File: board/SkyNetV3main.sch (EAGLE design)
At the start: 67 parts, among them IC1 HC_05, IC2 RF4463PRO, IC3 LPC1768, IC4 BCX17, IC5 TPS63001, IC6 MCP73871-2CCI/ML, Q1 32.768KHz, Q2 12MHz, Q3 IRLM6402, Q4 BSS138, X1 BAT

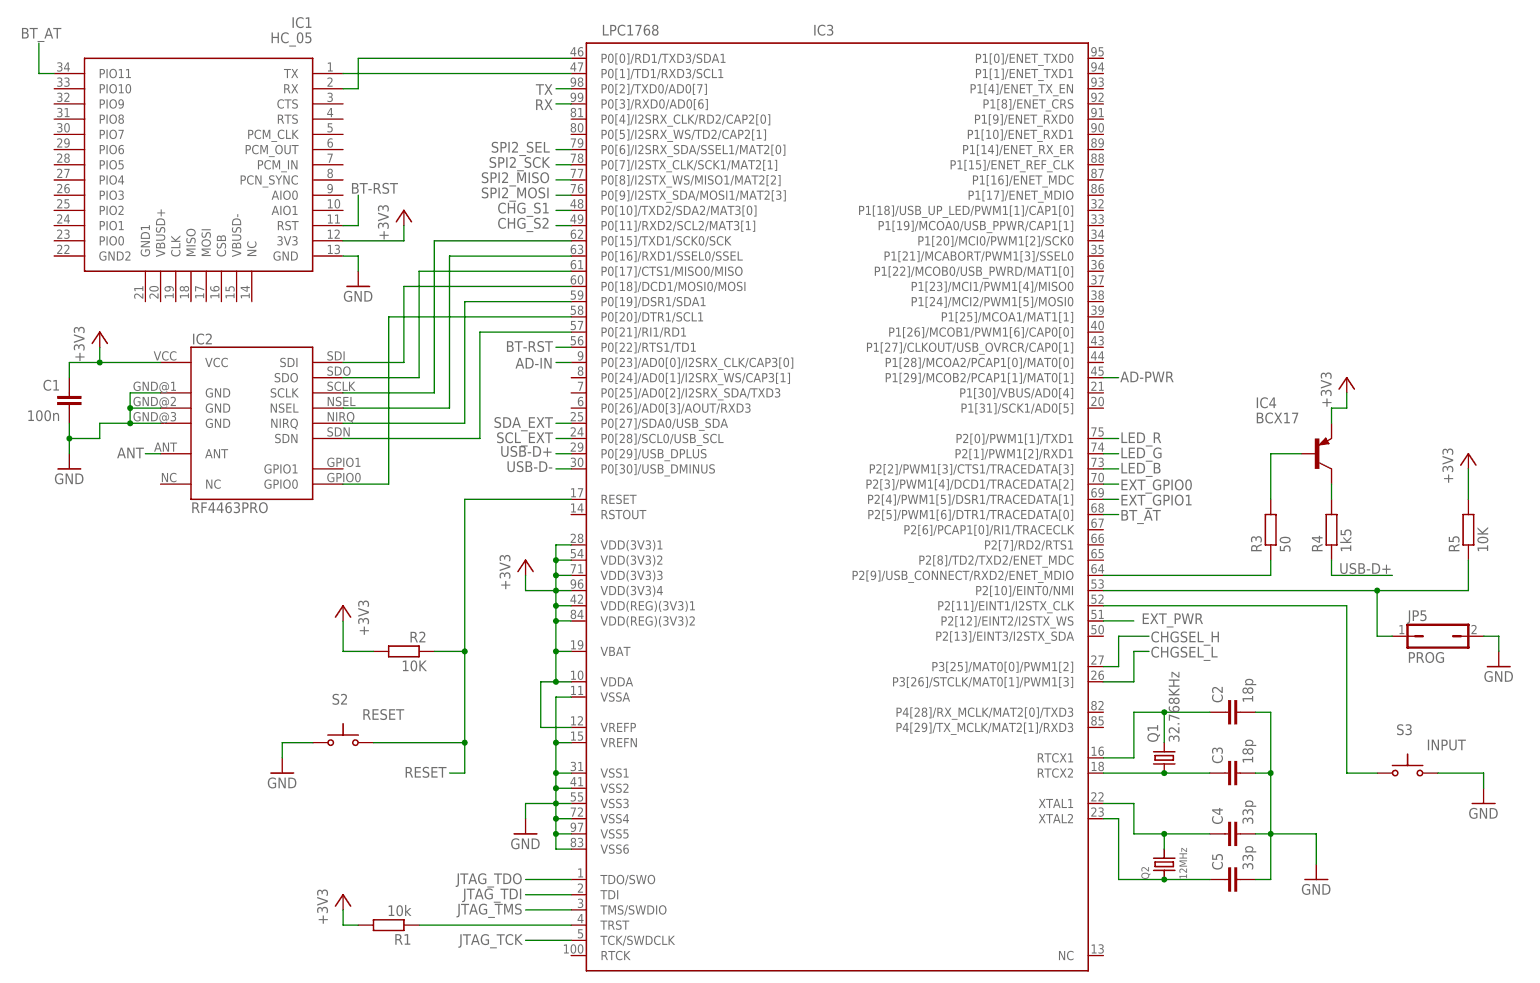
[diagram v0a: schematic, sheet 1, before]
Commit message: new layout
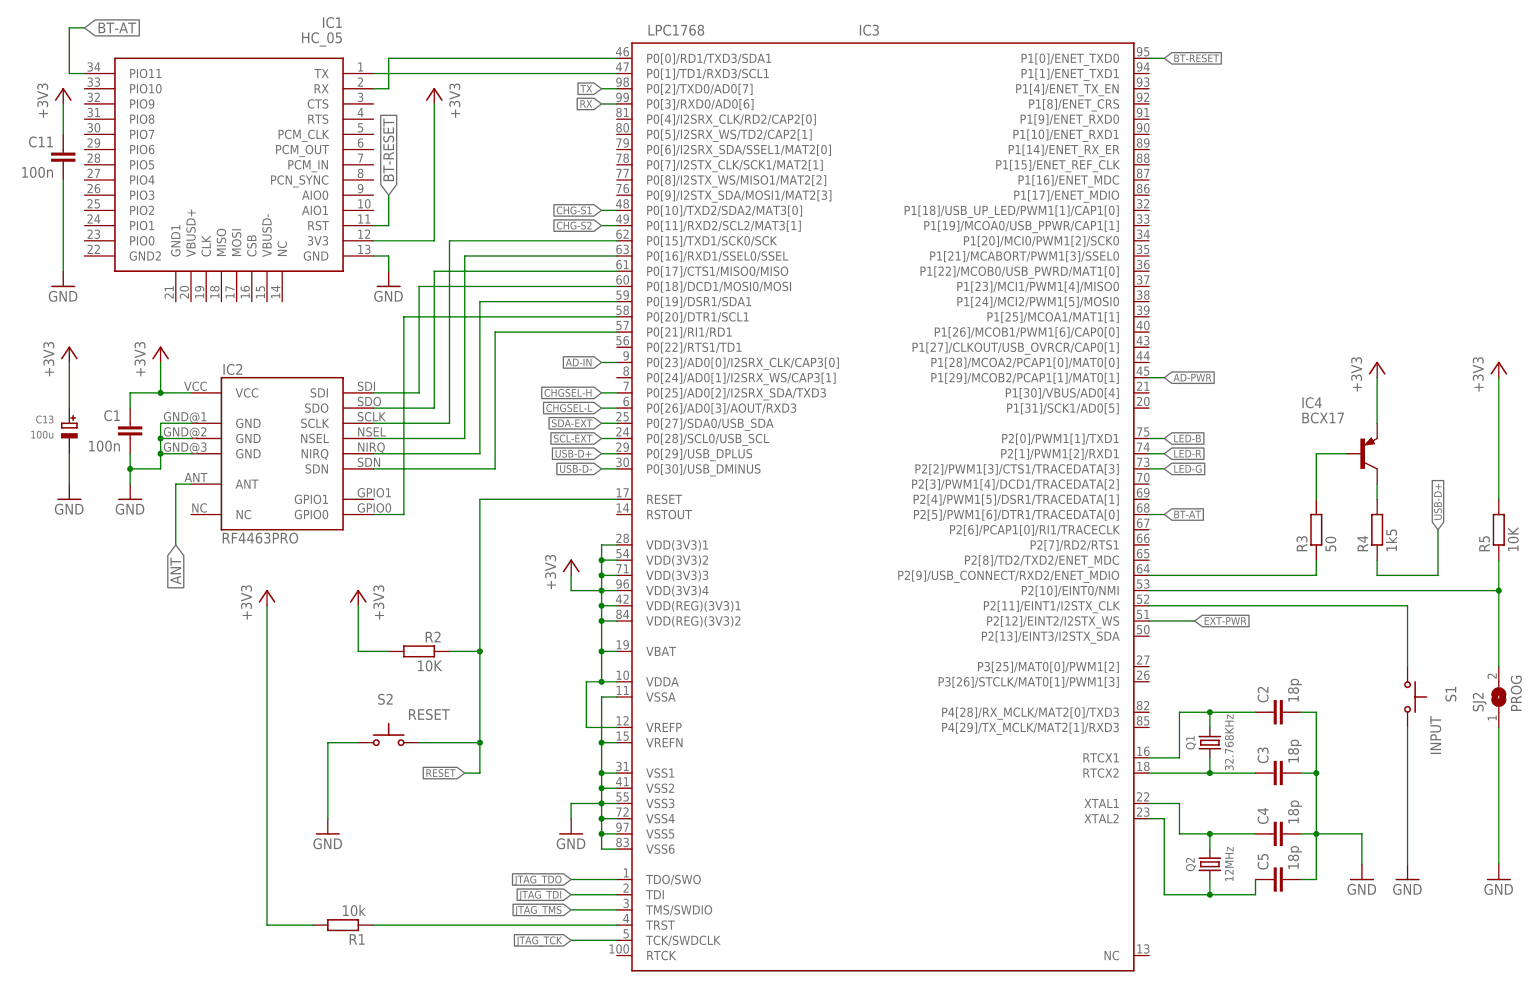
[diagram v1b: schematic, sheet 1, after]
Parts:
- removed C14: 100n, rcl:C-EUC0603
- removed JP1: MEASURE, jumper:JP1Q
- removed JP2: DEBUG, pinhead:PINHD-1X5
- removed JP4: PERIPH, microbuilder:HEADER-2X51.27MM
- removed JP5: PROG, jumper:JP1Q
- removed LED1: STATUS, skynet_other:RGB-LED
- removed OK1, OK2, OK3: PC3H7, skynet_other:PC3H7
- removed R7, R8: 91, rcl:R-EU_R0603
- removed S3: INPUT, skynet_other:PT645VERT
- added D1: 3v3, diode:ZENER-DIODESOT23
- added LED2: RGBLED5050, adafruit:RGBLED5050
- added S1: INPUT, switch-ck:PTS645SSMTR
- added SJ1: (no value), jumper:SJ
- added SJ2: PROG, jumper:SJ
- added U$2: (no value), skynet_other:PIN-HEAD-1X3
- C12, C13: value 100n -> 100u; device rcl:C-EUC0603 -> microbuilder:CAP_TANTALUMC/6032_WAVE
- C4, C5: value 33p -> 18p
- Q1: device crystal-2:CRYSTALMM20SS -> skynet_other:XTAL2-PAD
- Q2: device microbuilder:CRYSTALSMD -> skynet_other:XTAL4-PAD
- R6: value 91 -> 10k
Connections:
- net BT_AT renamed BT-AT
- net BT_RX renamed BT-RX
- net BT_TX renamed BT-TX
- net RTCX2 renamed N$2
- net SDI renamed RF-SDI
- net SPI0-NIRQ renamed RF-NIRQ
- net SPI0-NSEL renamed RF-NSEL
- net SPI0-SCLK renamed RF-SCLK
- net SPI0-SDN renamed RF-SDN
- net SPI0-SDO renamed RF-SDO
- removed net BT-RST: IC1.RST, IC3.P0[22]/RTS1/TD1
- removed net CHGSEL_H: IC3.P3[25]/MAT0[0]/PWM1[2], IC6.SEL
- removed net CHGSEL_L: IC3.P3[26]/STCLK/MAT0[1]/PWM1[3], IC6.PROG2
- removed net CHG_S1: IC3.P0[10]/TXD2/SDA2/MAT3[0], OK3.COL
- removed net CHG_S2: IC3.P0[11]/RXD2/SCL2/MAT3[1], OK2.COL
- removed net EXT_GPIO0: IC3.P2[3]/PWM1[4]/DCD1/TRACEDATA[2], JP4.6
- removed net EXT_GPIO1: IC3.P2[4]/PWM1[5]/DSR1/TRACEDATA[1], JP4.8
- removed net EXT_PWR: IC3.P2[12]/EINT2/I2STX_WS, OK1.COL
- removed net LED_B: IC3.P2[2]/PWM1[3]/CTS1/TRACEDATA[3], LED1-B.C
- removed net LED_G: IC3.P2[1]/PWM1[2]/RXD1, LED1-G.C
- removed net LED_R: IC3.P2[0]/PWM1[1]/TXD1, LED1-R.C
- removed net PG: IC6./PG, R6.1
- removed net PG-OK: OK1.C, R6.2
- removed net SCL_EXT: IC3.P0[28]/SCL0/USB_SCL, JP4.4
- removed net SDA_EXT: IC3.P0[27]/SDA0/USB_SDA, JP4.2
- removed net SPI2_MISO: IC3.P0[8]/I2STX_WS/MISO1/MAT2[2], JP4.5
- removed net SPI2_MOSI: IC3.P0[9]/I2STX_SDA/MOSI1/MAT2[3], JP4.7
- removed net SPI2_SCK: IC3.P0[7]/I2STX_CLK/SCK1/MAT2[1], JP4.3
- removed net SPI2_SEL: IC3.P0[6]/I2SRX_SDA/SSEL1/MAT2[0], JP4.1
- removed net STAT1: IC6.STAT1/LBO, R8.1
- removed net STAT1-OK: OK3.C, R8.2
- removed net STAT2: IC6.STAT2, R7.1
- removed net STAT2-OK: OK2.C, R7.2
- new net BT-RESET: IC1.RST, IC3.P1[0]/ENET_TXD0
- new net CHG-S1: IC3.P0[10]/TXD2/SDA2/MAT3[0], IC6.STAT1/LBO
- new net CHG-S2: IC3.P0[11]/RXD2/SCL2/MAT3[1], IC6.STAT2
- new net CHGSEL-H: IC3.P0[25]/AD0[2]/I2SRX_SDA/TXD3, IC6.SEL
- new net CHGSEL-L: IC3.P0[26]/AD0[3]/AOUT/RXD3, IC6.PROG2
- new net EXT-PWR: D1.C, IC3.P2[12]/EINT2/I2STX_WS, R6.2
- new net LED-B: IC3.P2[0]/PWM1[1]/TXD1, LED2.BLUE_C
- new net LED-G: IC3.P2[2]/PWM1[3]/CTS1/TRACEDATA[3], LED2.GREEN_C
- new net LED-R: IC3.P2[1]/PWM1[2]/RXD1, LED2.RED_C
- new net SCL-EXT: IC3.P0[28]/SCL0/USB_SCL, U$2.4
- new net SDA-EXT: IC3.P0[27]/SDA0/USB_SDA, U$2.3
- net +3V3: now also C12.+, C13.+, U$2.5; no longer C12.1, C13.1, C14.1, JP2.4, JP4.10
- net +5V: now also R6.1; no longer OK1.A, OK2.A, OK3.A
- net GND: now also C12.-, C13.-, D1.A, S1.S, SJ2.1, U$2.6; no longer C12.2, C13.2, C14.2, JP2.5, JP4.9, JP5.2, OK1.EMI, OK2.EMI, OK3.EMI, S3.S
- net INPUT: now also S1.P; no longer S3.P
- net LED-B-R: now also LED2.BLUE_A; no longer LED1-B.A
- net LED-G-R: now also LED2.GREEN_A; no longer LED1-G.A
- net LED-R-R: now also LED2.RED_A; no longer LED1-R.A
- net OUT2: now also SJ1.1; no longer JP1.1
- net PROG: now also SJ2.2; no longer JP5.1
- net RX: now also U$2.1; no longer JP2.1
- net TX: now also U$2.2; no longer JP2.3
- net VCC: now also SJ1.2; no longer JP1.2
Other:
- note added: "tantal fehlen"
- moved on the sheet: C1, C10, C15, C2, C3, C4, C5, C9, IC1, IC2, IC3, IC4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
